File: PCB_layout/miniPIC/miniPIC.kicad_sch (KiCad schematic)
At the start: 41 parts, among them J1 Conn_01x09, J2 Conn_01x06, J3 Conn_01x10, J4 Conn_01x08, J5 Jack-DC, J6 Conn_01x05, J7 Conn_01x04, J9 USB_B_Mini, SW1 EG2201B, U1 PIC16F887-IP, U2 AMS1117-3.3, U3 78M05, Y1 Crystal

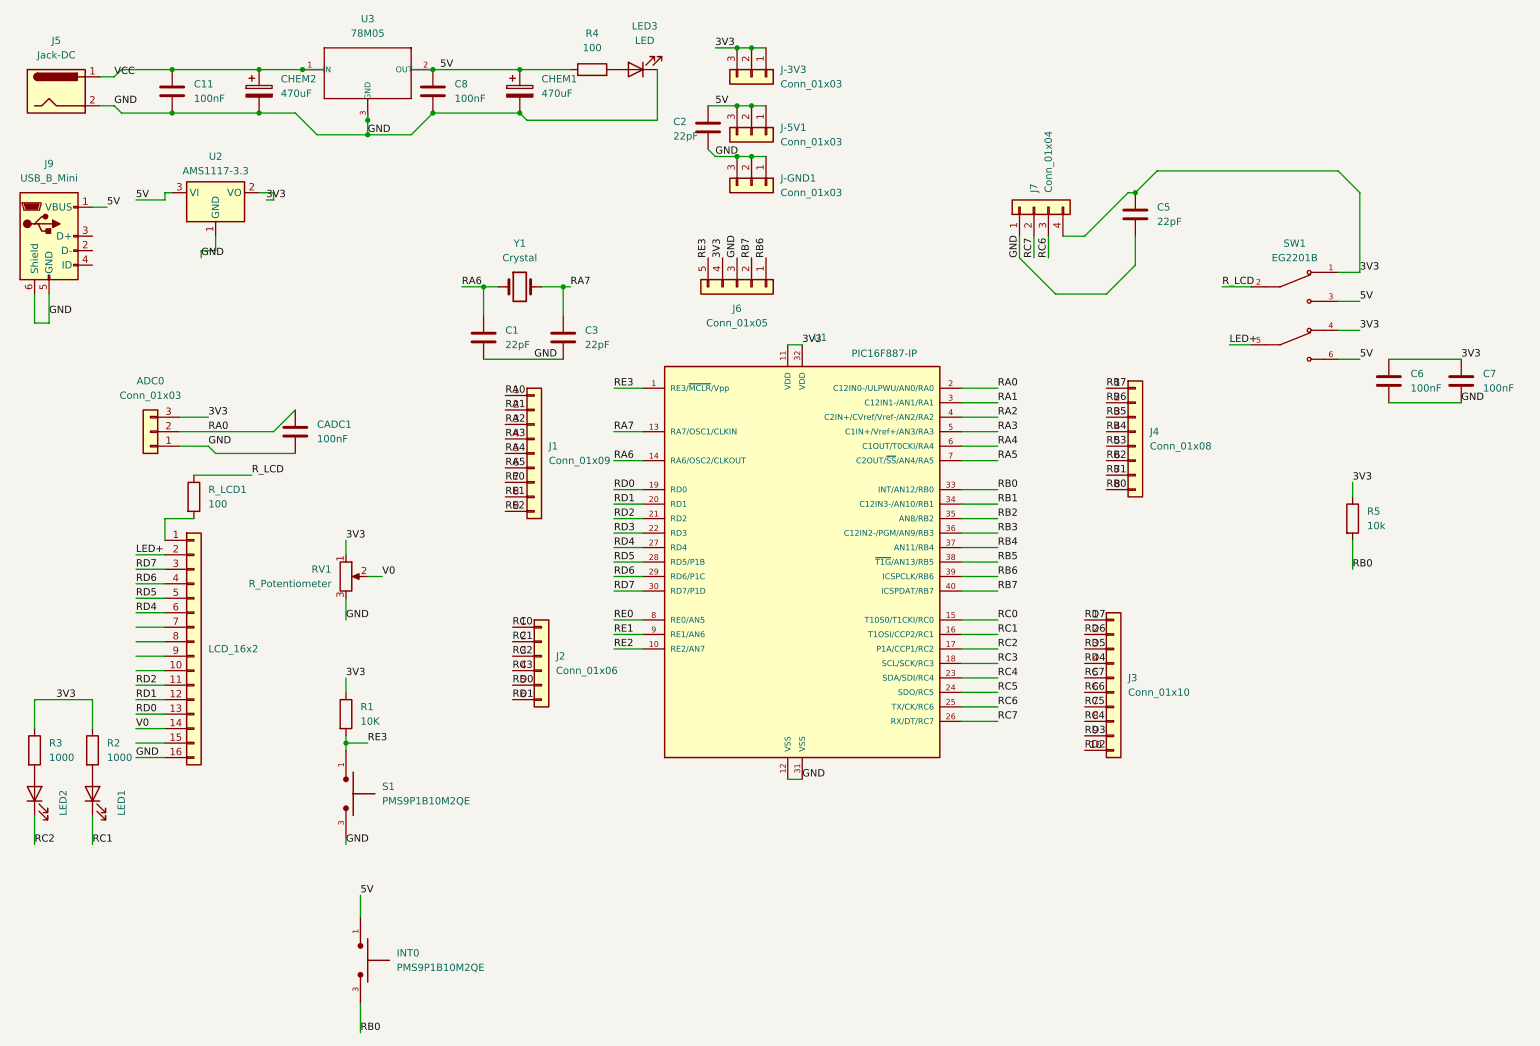
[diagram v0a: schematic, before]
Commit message: add: PCB_layout
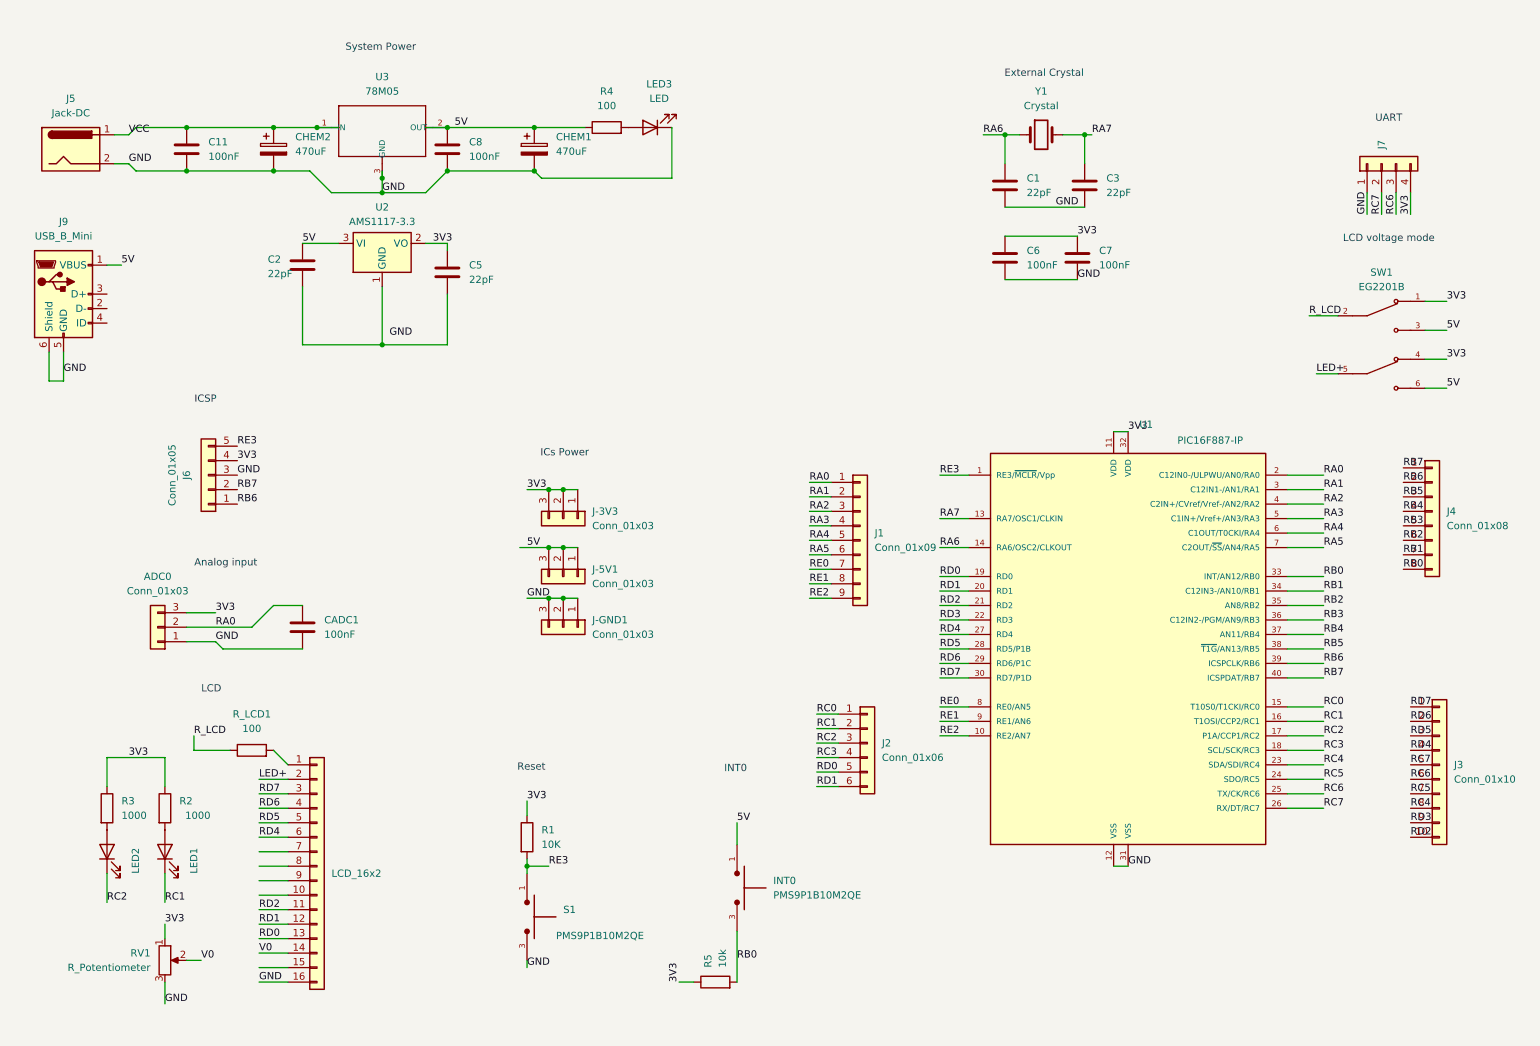
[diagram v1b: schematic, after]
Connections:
- net GND: no longer C2.2, C5.2, U2.1 (GND)
- new net: C2.2, C5.2, U2.1 (GND)
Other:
- note added: "Analog input"
- note added: "External Crystal"
- note added: "ICSP"
- note added: "ICs Power"
- note added: "INT0"
- note added: "LCD"
- note added: "LCD voltage mode"
- note added: "Reset"
- note added: "System Power"
- note added: "UART"
- moved on the sheet: ADC0, C1, C11, C2, C3, C5, C6, C7, C8, CADC1, CHEM1, CHEM2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
